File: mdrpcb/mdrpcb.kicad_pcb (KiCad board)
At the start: 2 copper layers, 91.4 x 76.2 mm, 38 parts, among them J1 Conn_02x04_Odd_Even, J10 Conn_01x06, J11 Conn_01x06, J2 Conn_01x03, J3 SM04B-SRSS-TB, J4 Conn_01x03, J5 Conn_01x03, J6 Conn_01x03, J7 Conn_01x03, J8 Conn_01x03, J9 Conn_01x06, SW1 SW_Push, SW2 SW_Push, SW3 SW_Push, SW4 SW_Push, U1 SC0918

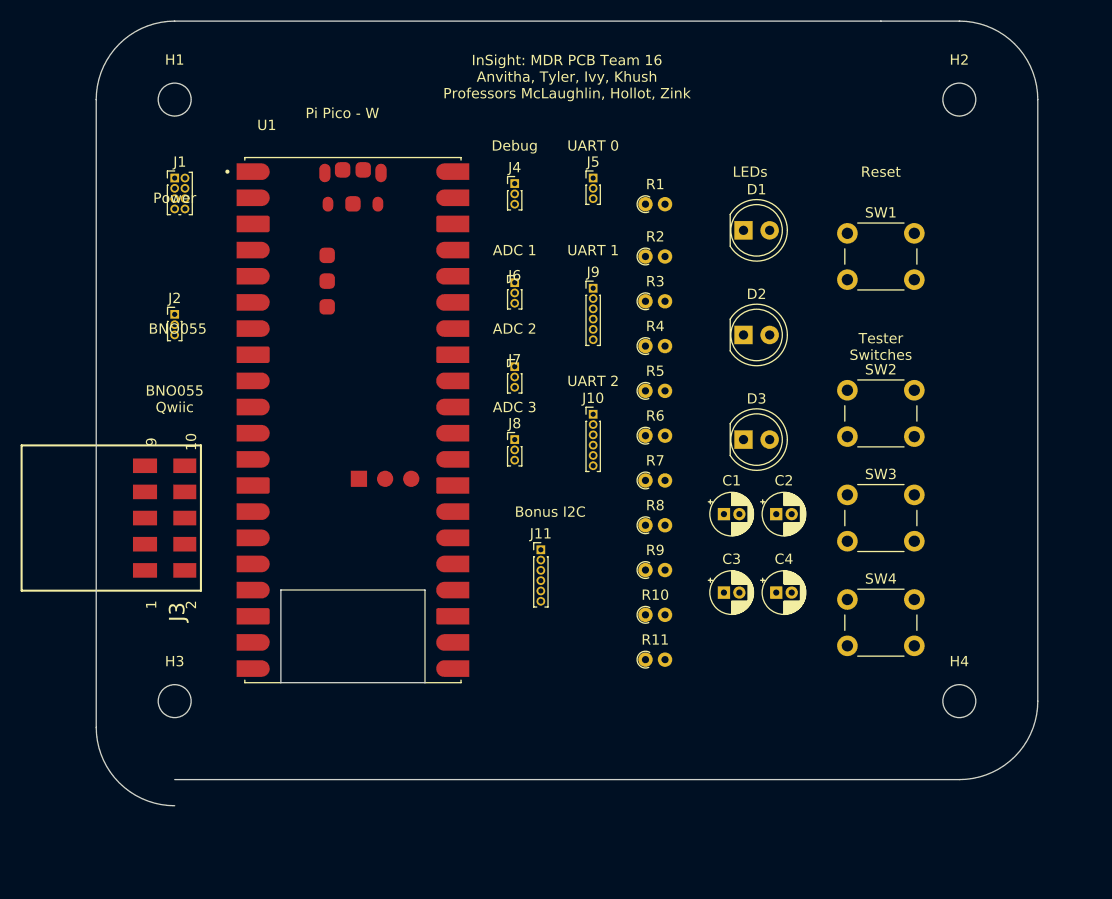
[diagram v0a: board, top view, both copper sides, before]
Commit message: Add files via upload
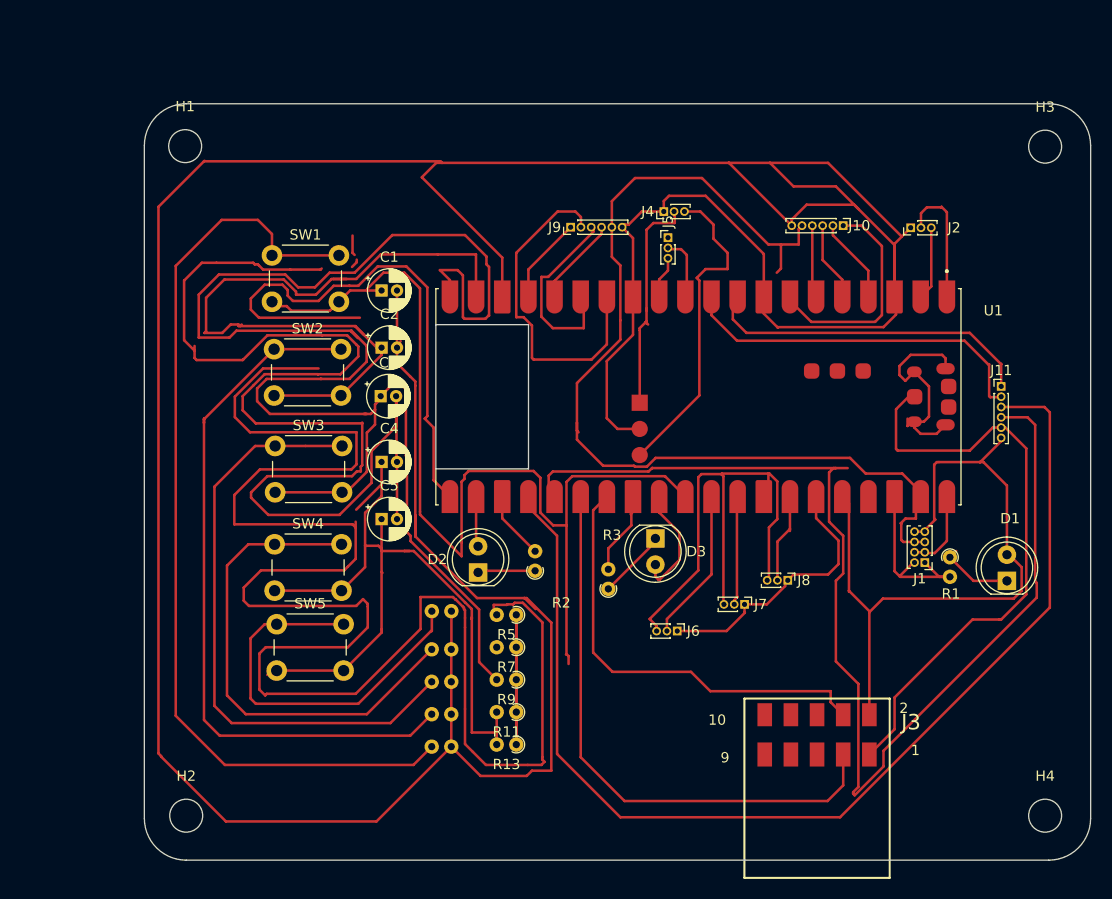
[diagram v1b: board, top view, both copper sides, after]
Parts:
- added C5: 100nF, Capacitor_THT:CP_Radial_D4.0mm_P1.50mm, F.Cu at (53.1, 68.7)
- added R12: 100, Resistor_THT:R_Axial_DIN0204_L3.6mm_D1.6mm_P1.90mm_Vertical, B.Cu at (58.0, 77.6)
- added R13: 10k, Resistor_THT:R_Axial_DIN0204_L3.6mm_D1.6mm_P1.90mm_Vertical, F.Cu at (66.2, 90.6)
- added SW5: SW_Push, Button_Switch_THT:SW_PUSH_6mm, F.Cu at (42.9, 78.9)
- R10, R4, R6, R8: moved to B.Cu
- moved H2 102.3 mm to (34.1, 97.5)
- moved H3 100.2 mm to (117.6, 32.5)
- moved J1 81.9 mm to (105.9, 72.9), turned to 180 degrees
- moved J3 78.6 mm to (95.4, 98.8), turned to 180 degrees
- moved J2 72.0 mm to (104.5, 40.4), turned to 90 degrees
- moved SW1 55.9 mm to (42.5, 43.1)
- moved SW4 55.9 mm to (42.7, 71.1)
- moved SW2 55.8 mm to (42.7, 52.2)
- moved SW3 55.8 mm to (42.8, 61.6)
- moved J11 47.4 mm to (113.3, 55.8)
- moved R1 45.3 mm to (108.3, 72.4), turned to -90 degrees
- moved R4 44.1 mm to (58.0, 90.8)
- moved D1 42.6 mm to (113.8, 74.7), turned to 90 degrees
- moved C2 41.6 mm to (53.1, 52.0)
- moved C4 40.4 mm to (53.1, 63.1)
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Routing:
- net GND: track 0.00 -> 588.4 mm
- net /RST: track 0.00 -> 269.1 mm
- net /SW1: track 0.00 -> 152.5 mm
- net /SW2: track 0.00 -> 133.5 mm
- net /I2C1_SCL: track 0.00 -> 112.8 mm
- net /I2C1_SDA: track 0.00 -> 108.9 mm
- net +5V: track 0.00 -> 97.5 mm
- net Net-(R4-Pad1): track 0.00 -> 91.6 mm
- net /SW0: track 0.00 -> 71.9 mm
- net Net-(R6-Pad1): track 0.00 -> 69.4 mm
- net +3.3V: track 0.00 -> 68.3 mm
- net Net-(R8-Pad1): track 0.00 -> 58.8 mm
- net /I2C0_SDA: track 0.00 -> 56.6 mm
- net GNDA: track 0.00 -> 50.7 mm
- net Net-(R10-Pad1): track 0.00 -> 47.8 mm
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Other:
- board size 91.4 x 76.2 mm -> 91.9 x 73.5 mm
- board text removed: "ADC 1"
- board text removed: "ADC 2"
- board text removed: "ADC 3"
- board text removed: "BNO055"
- board text removed: "BNO055 Qwiic"
- board text removed: "Bonus I2C"
- board text removed: "Debug"
- board text removed: "InSight: MDR PCB Team 16 Anvitha, Tyler, Ivy, Khush Professors McLaughlin, Hollot, Zink"
- board text removed: "LEDs"
- board text removed: "Pi Pico - W"
- board text removed: "Power"
- board text removed: "Reset"
- board text removed: "Tester Switches"
- board text removed: "UART 0"
- board text removed: "UART 1"
- board text removed: "UART 2"

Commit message: Add files via upload
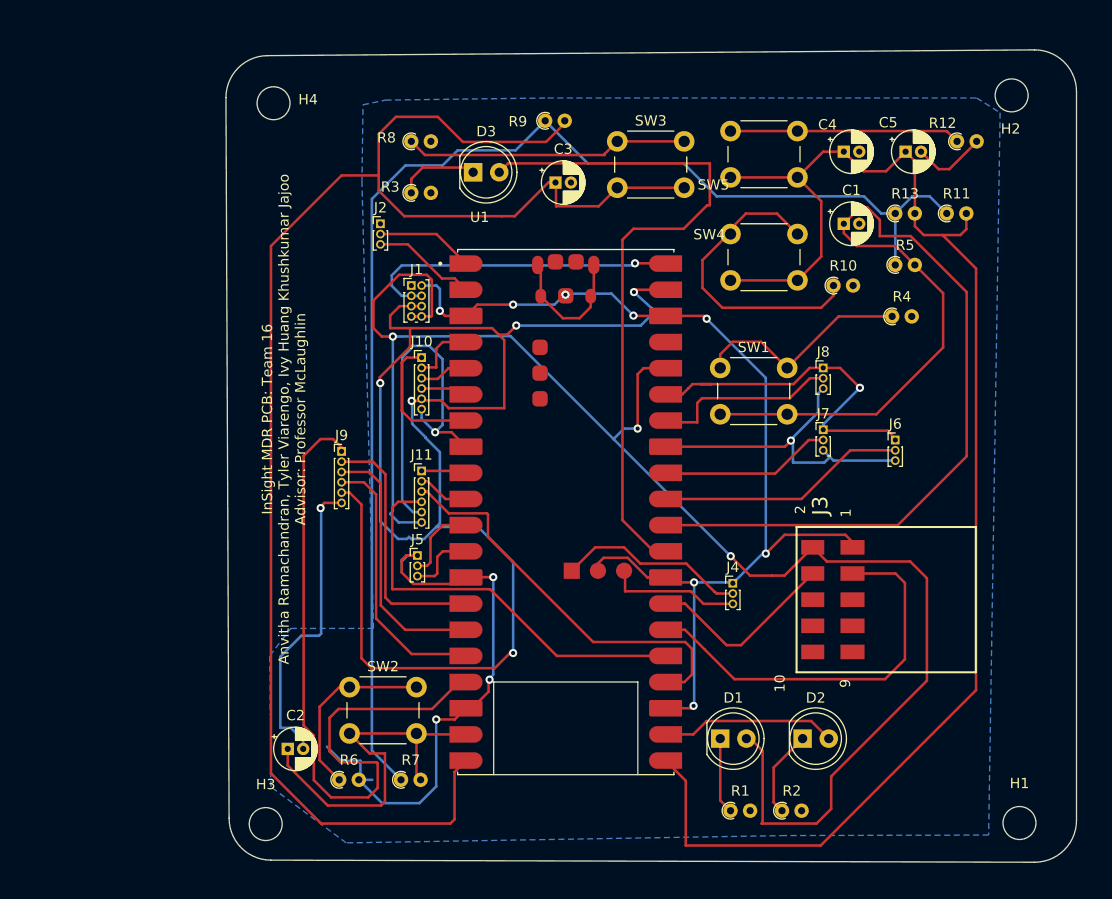
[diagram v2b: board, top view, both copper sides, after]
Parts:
- R10, R12, R4, R6, R8: moved to F.Cu
- moved H2 106.4 mm to (114.3, 27.5)
- moved H1 104.3 mm to (115.1, 98.2)
- moved H4 102.0 mm to (42.6, 28.3)
- moved H3 100.3 mm to (41.9, 98.3)
- moved R12 68.4 mm to (109.0, 32.0)
- moved SW5 65.1 mm to (87.0, 31.0)
- moved R11 64.0 mm to (108.0, 39.0), turned to 0 degrees
- moved R13 63.4 mm to (103.0, 39.0), turned to 0 degrees
- moved C5 62.2 mm to (104.0, 33.0)
- moved R4 61.2 mm to (102.7, 49.0)
- moved J11 56.9 mm to (57.0, 64.0)
- moved J1 56.7 mm to (56.0, 46.0), turned to 0 degrees
- moved R9 54.3 mm to (69.0, 30.0), turned to 0 degrees
- moved C4 54.1 mm to (98.0, 33.0)
- moved SW4 53.6 mm to (87.0, 41.0)
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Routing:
- net GND: track 588.4 -> 229.4 mm, vias 0 -> 13
- net /RST: track 269.1 -> 107.5 mm
- net +3V3: track 25.2 -> 126.7 mm
- net +3.3V: track 68.3 -> 155.6 mm, vias 0 -> 3
- net /I2C1_SCL: track 112.8 -> 40.2 mm
- net Net-(R4-Pad1): track 91.6 -> 20.9 mm
- net /I2C1_SDA: track 108.9 -> 39.2 mm
- net /SPI1_CS: track 8.47 -> 69.7 mm
- net /LED1: track 13.0 -> 67.4 mm
- net Net-(R6-Pad1): track 69.4 -> 18.1 mm
- net +5V: track 97.5 -> 145.1 mm, vias 0 -> 5
- net /SW0: track 71.9 -> 37.8 mm
- net Net-(R8-Pad1): track 58.8 -> 27.7 mm
- net /GP7_AD0: track 35.0 -> 5.03 mm
- net /GP6_INT: track 32.4 -> 4.39 mm
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- added copper zone on B.Cu, net GND
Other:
- board size 91.9 x 73.5 mm -> 82.6 x 78.9 mm
- board text added: "InSight MDR PCB: Team 16 Anvitha Ramachandran, Tyler Viarengo, Ivy Huang Khushkumar Jajoo Advisor: Professor McLaughlin"
